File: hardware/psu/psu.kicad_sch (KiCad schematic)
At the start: 58 parts, among them J1 Conn_01x02, J10 Conn_01x04, J11 Conn_01x03, J12 Conn_01x02, J13 Conn_01x03, J14 Conn_01x05, J2 Conn_01x05, J3 Conn_01x02, J4 Conn_01x06, J5 Conn_01x03, J6 Conn_01x05, J7 Conn_01x08, J8 Conn_01x03, J9 Conn_01x04, SW1 SW_SPST, T1 AS-1T175, U1 LM7905_TO220

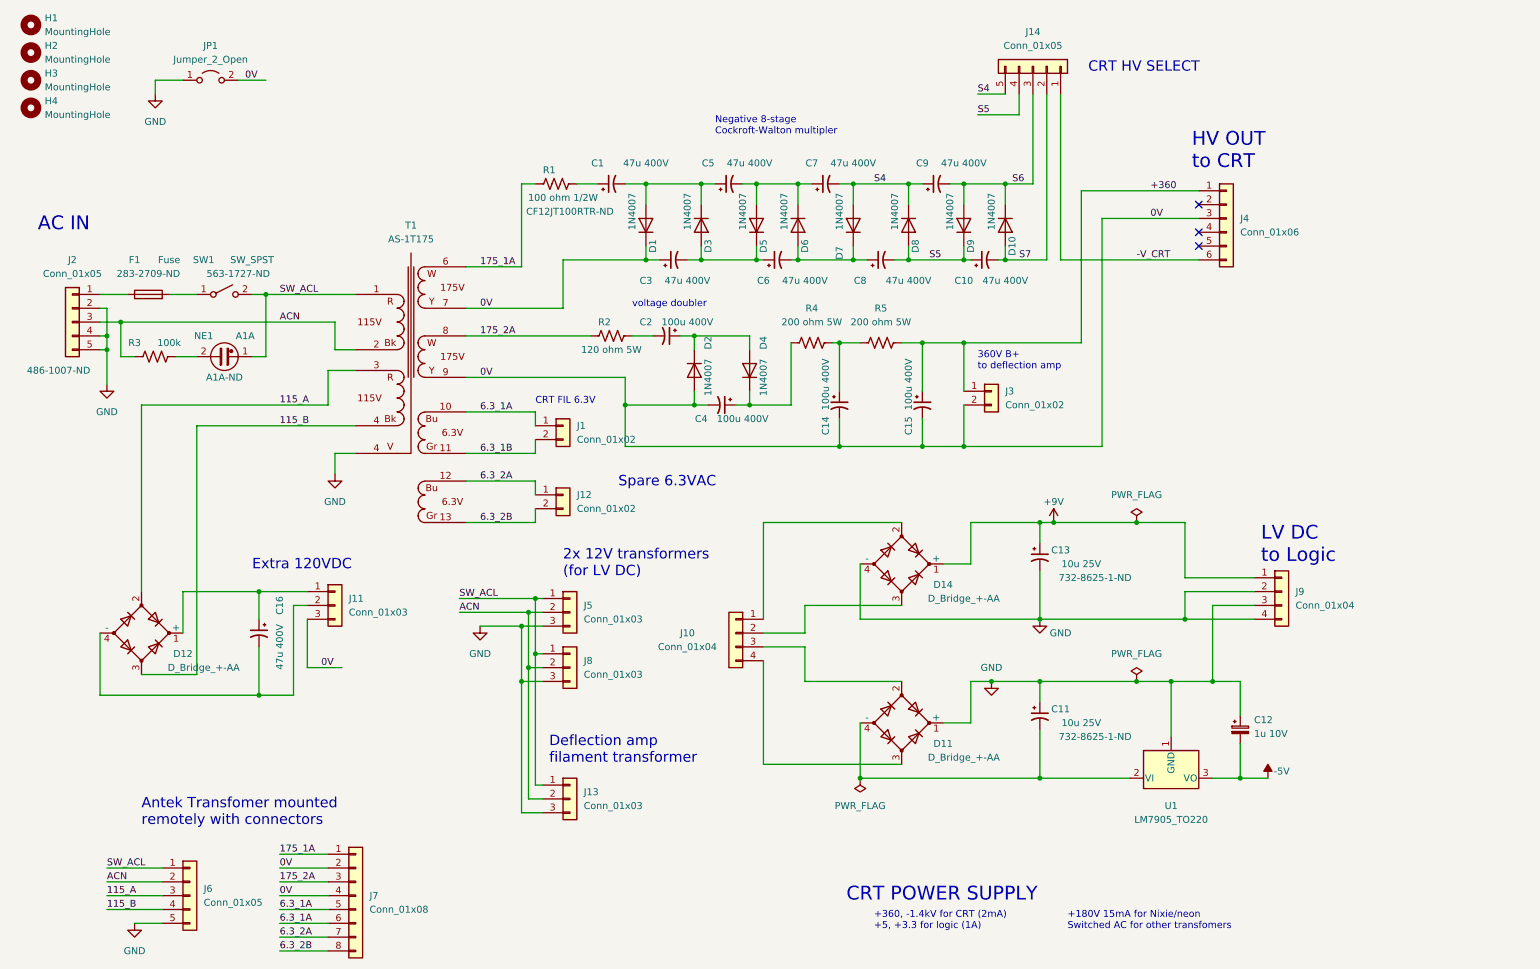
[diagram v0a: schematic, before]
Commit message: working on PSU
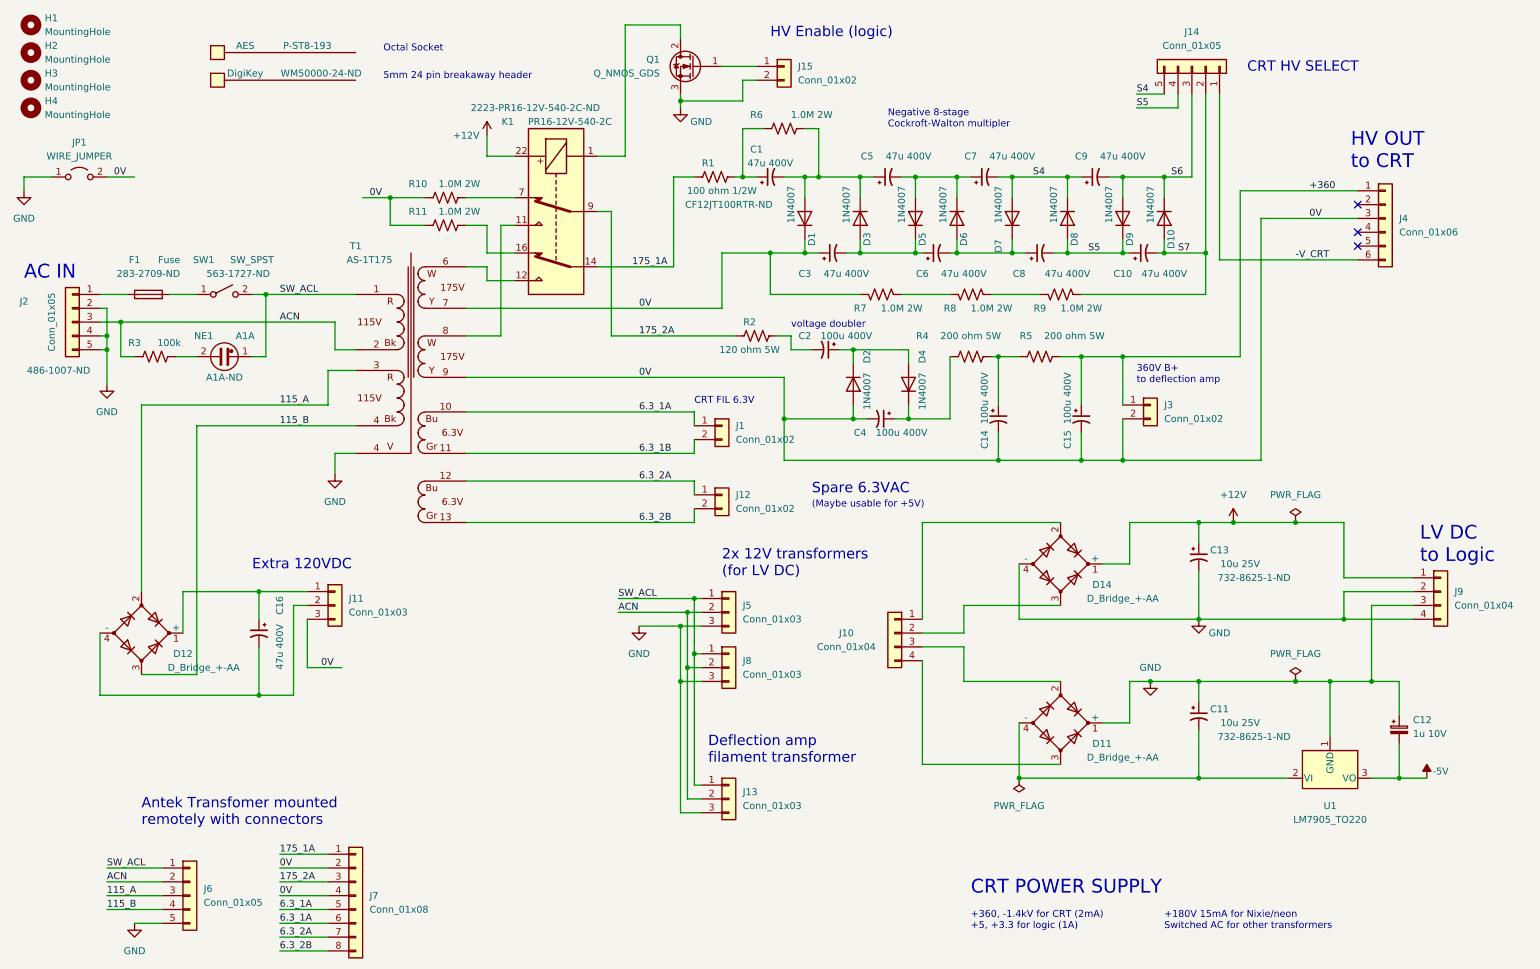
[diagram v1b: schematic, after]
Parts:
- added J15: Conn_01x02, Connector_PinHeader_2.54mm:PinHeader_1x02_P2.54mm_Vertical, symbol Connector_Generic:Conn_01x02
- added K1: PR16-12V-540-2C, Package_DIP:DIP-22_W7.62mm_LongPads, symbol my_relay:PR16-12V-540-2A
- added Q1: Q_NMOS_GDS, Package_TO_SOT_THT:TO-220-3_Vertical, symbol Device:Q_NMOS_GDS
- added R10, R11, R6, R7, R8, R9: 1.0M 2W, Resistor_THT:R_Axial_DIN0309_L9.0mm_D3.2mm_P15.24mm_Horizontal, symbol Device:R_US
- added U2, U3: BOM_item, symbol misc_bom:BOM_item
- C1, C10, C16, C3, C5, C6, C7, C8, C9: footprint Capacitor_THT:CP_Radial_D13.0mm_P7.50mm -> Capacitor_THT:CP_Radial_D12.5mm_P5.00mm; CatNo (none) -> 565-EKXJ401ELL470MK30S-ND
- C12: footprint Capacitor_THT:CP_Radial_D5.0mm_P2.00mm -> Capacitor_THT:C_Disc_D5.0mm_W2.5mm_P5.00mm; CatNo (none) -> 445-FK28X5R1A105K-ND
- C14, C15, C2, C4: CatNo (none) -> 493-2567-ND
- JP1: value Jumper_2_Open -> WIRE_JUMPER
- R2: footprint Resistor_THT:R_Axial_Power_L25.0mm_W6.4mm_P27.94mm -> Resistor_THT:R_Axial_DIN0617_L17.0mm_D6.0mm_P25.40mm_Horizontal; CatNo (none) -> A142778CT-ND
- R4, R5: footprint Resistor_THT:R_Axial_Power_L25.0mm_W6.4mm_P27.94mm -> Resistor_THT:R_Axial_DIN0617_L17.0mm_D6.0mm_P25.40mm_Horizontal; CatNo (none) -> A142783CT-ND
- U1: CatNo (none) -> LM7905CTNS/NOPB-ND
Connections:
- net 0V: now also R10.1, R11.1, R7.1
- net 175_1A: now also K1.14; no longer T1.6 (H1A)
- net 175_2A: now also K1.9; no longer T1.8 (H2A)
- net GND: now also J15.2 (Pin_2), Q1.3 (S)
- net S7: now also R9.2
- net at C1.2, C5.1, D1.2 (A)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: now also R6.2
- net at C1.1, R1.2: now also R6.1
- net +9V renamed +12V
- net +12V: now also K1.22
- new net: K1.1, Q1.2 (D)
- new net: K1.11, T1.8 (H2A)
- new net: K1.12, T1.6 (H1A)
- new net: K1.16, R11.2
- new net: K1.7, R10.2
- new net: R7.2, R8.1
- new net: J15.1 (Pin_1), Q1.1 (G)
- new net: R8.2, R9.1
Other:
- note added: "(Maybe usable for +5V)"
- note added: "+180V 15mA for Nixie/neon Switched AC for other transformers"
- note added: "5mm 24 pin breakaway header"
- note added: "HV Enable (logic)"
- note added: "Octal Socket"
- note removed: "+180V 15mA for Nixie/neon Switched AC for other transfomers"
- moved on the sheet: C1, C10, C11, C12, C13, C14, C15, C2, C3, C4, C5, C6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
